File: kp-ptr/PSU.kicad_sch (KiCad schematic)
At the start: 21 parts, among them J2 Conn_01x02, J3 Conn_01x02

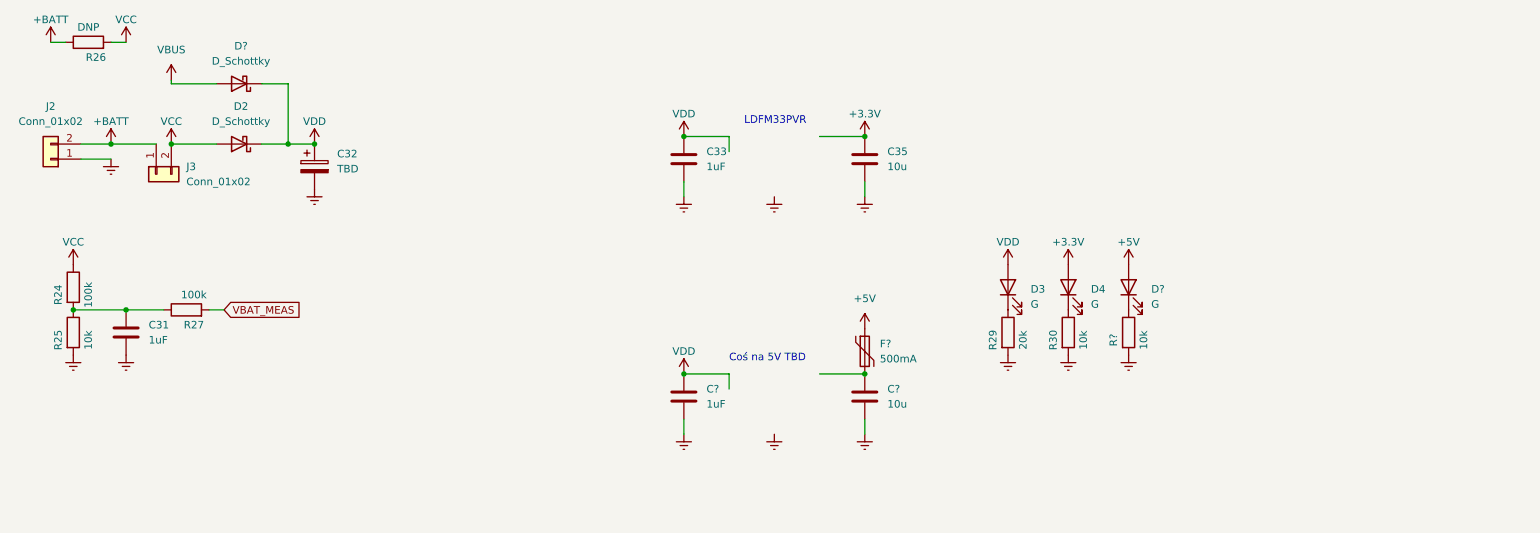
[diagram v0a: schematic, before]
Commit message: Update po spotkaniu
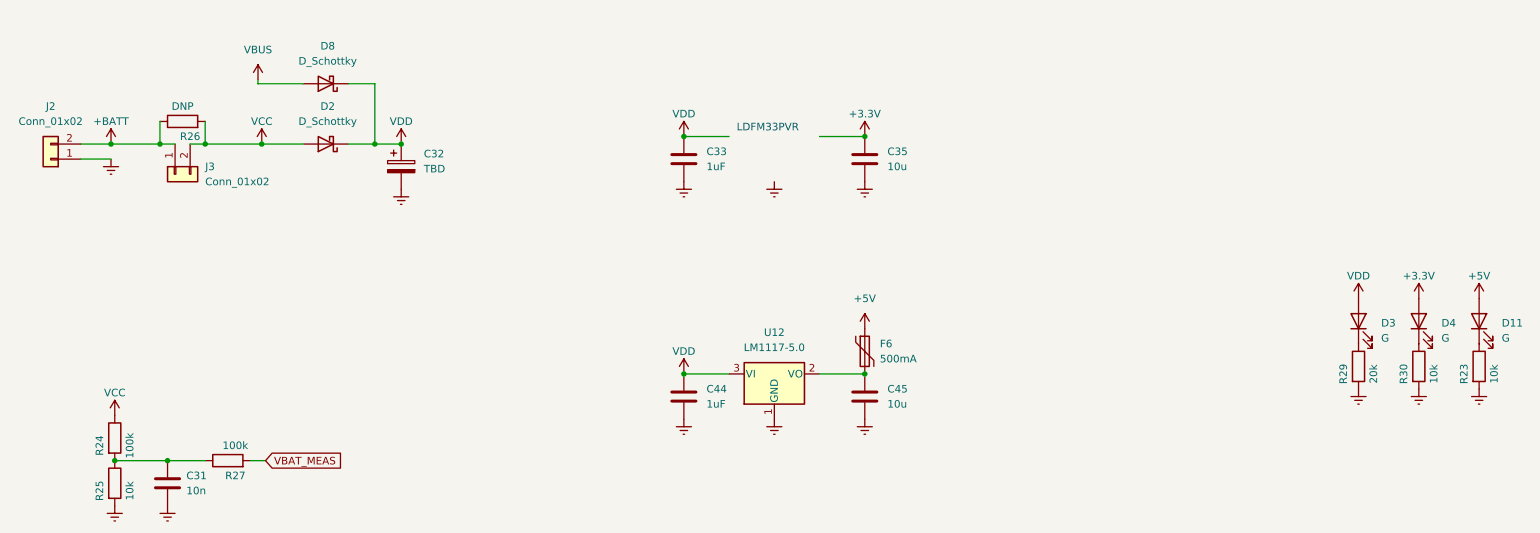
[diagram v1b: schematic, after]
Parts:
- added U12: LM1117-5.0, symbol Regulator_Linear:LM1117-5.0
- C31: value 1uF -> 10n; footprint Capacitor_SMD:C_0402_1005Metric_Pad0.74x0.62mm_HandSolder -> Capacitor_SMD:C_0402_1005Metric
- C32, C33, C35: footprint Capacitor_SMD:C_0402_1005Metric_Pad0.74x0.62mm_HandSolder -> Capacitor_SMD:C_0402_1005Metric
- C44, C45: renamed from C?; footprint Capacitor_SMD:C_0402_1005Metric_Pad0.74x0.62mm_HandSolder -> Capacitor_SMD:C_0402_1005Metric
- D11: renamed from D?; footprint LED_SMD:LED_0402_1005Metric_Pad0.77x0.64mm_HandSolder -> LED_SMD:LED_0603_1608Metric
- D3, D4: footprint LED_SMD:LED_0402_1005Metric_Pad0.77x0.64mm_HandSolder -> LED_SMD:LED_0603_1608Metric
- F6: renamed from F?; footprint Fuse:Fuse_1206_3216Metric_Pad1.42x1.75mm_HandSolder -> Fuse:Fuse_0805_2012Metric
- R23: renamed from R?; footprint Resistor_SMD:R_0402_1005Metric_Pad0.72x0.64mm_HandSolder -> Resistor_SMD:R_0402_1005Metric
- R24, R25, R26, R27, R29, R30: footprint Resistor_SMD:R_0402_1005Metric_Pad0.72x0.64mm_HandSolder -> Resistor_SMD:R_0402_1005Metric
- gave numbers to parts that had none: 1
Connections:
- net Earth: now also U12.1 (GND)
- net VDD: now also U12.3 (VI)
- net at C45.1, F6.2: now also U12.2 (VO)
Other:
- note removed: "Coś na 5V TBD"
- moved on the sheet: C31, C32, D11, D2, D3, D4, D8, J3, R23, R24, R25, R26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
